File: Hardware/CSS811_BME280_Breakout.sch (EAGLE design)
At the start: 35 parts, among them J1 GATORGATOR_MINI, J2 GATORGATOR_MINI, J3 GATORGATOR_MINI, J4 GATORGATOR_MINI, J5 GATORGATOR_MINI, J6 GATORGATOR_MINI, J7 GATORGATOR_MINI, J8 GATORGATOR_MINI, Q1 2.5A/30V/105mΩ, U2 CCS811, U3 BME280

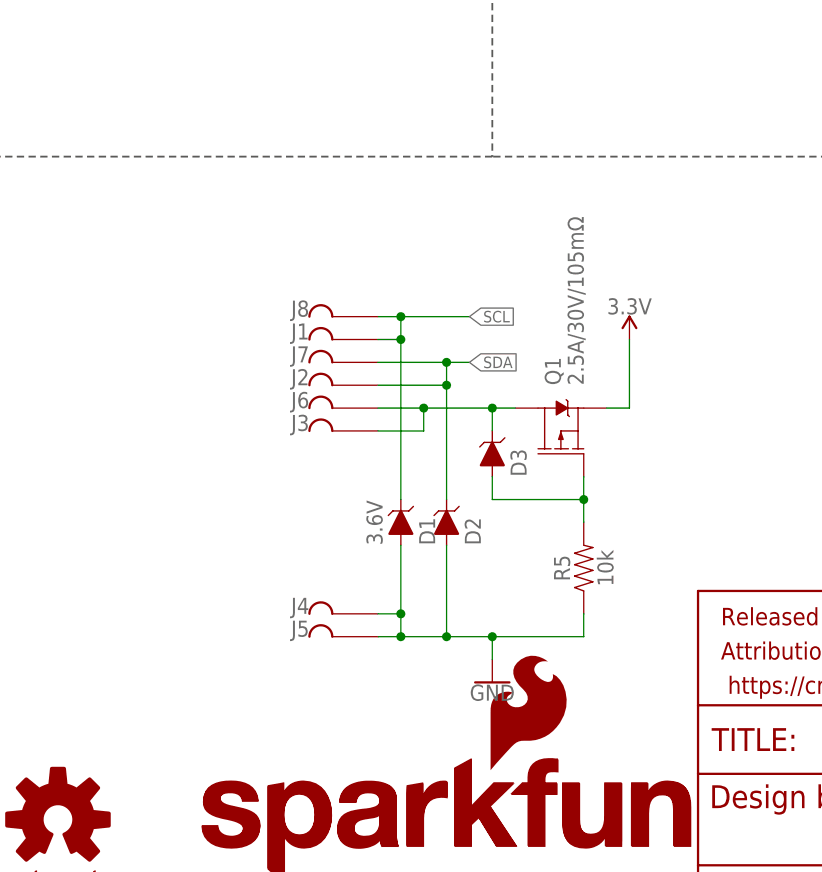
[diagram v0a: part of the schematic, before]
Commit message: pushing unsaved changes from checklist
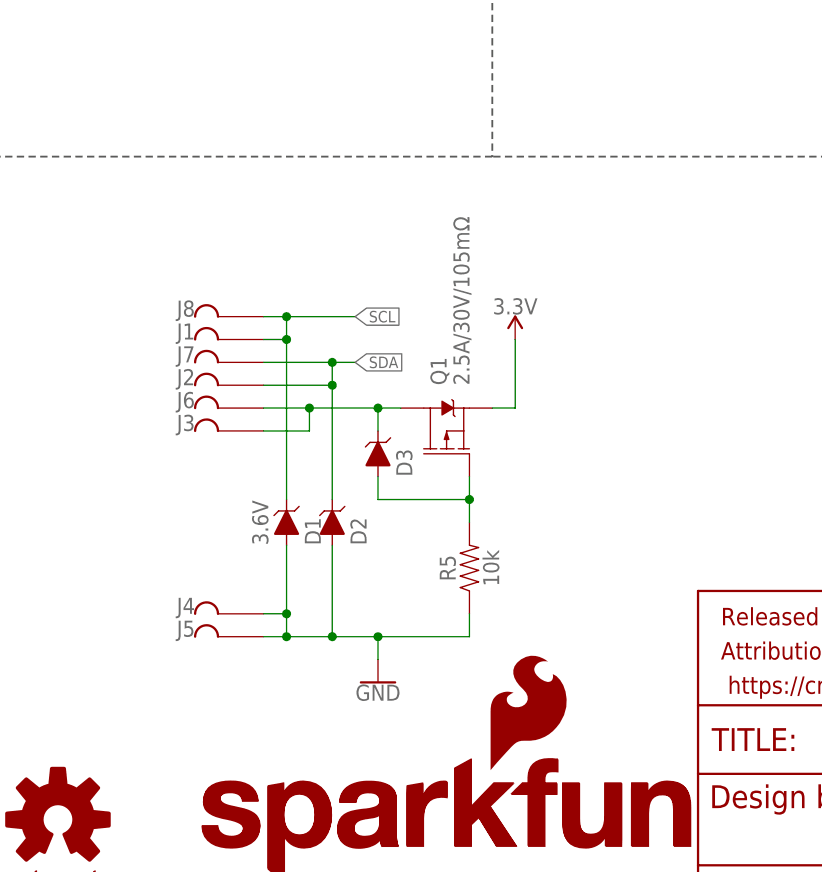
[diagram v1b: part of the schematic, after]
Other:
- moved on the sheet: D1, D2, D3, J1, J2, J3, J4, J5, J6, J7, J8, Q1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
